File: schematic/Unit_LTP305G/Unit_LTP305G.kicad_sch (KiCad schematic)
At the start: 15 parts, among them J1 Conn_01x04, U1 M5StampS3, U2 LTP305G, U3 LTR305G

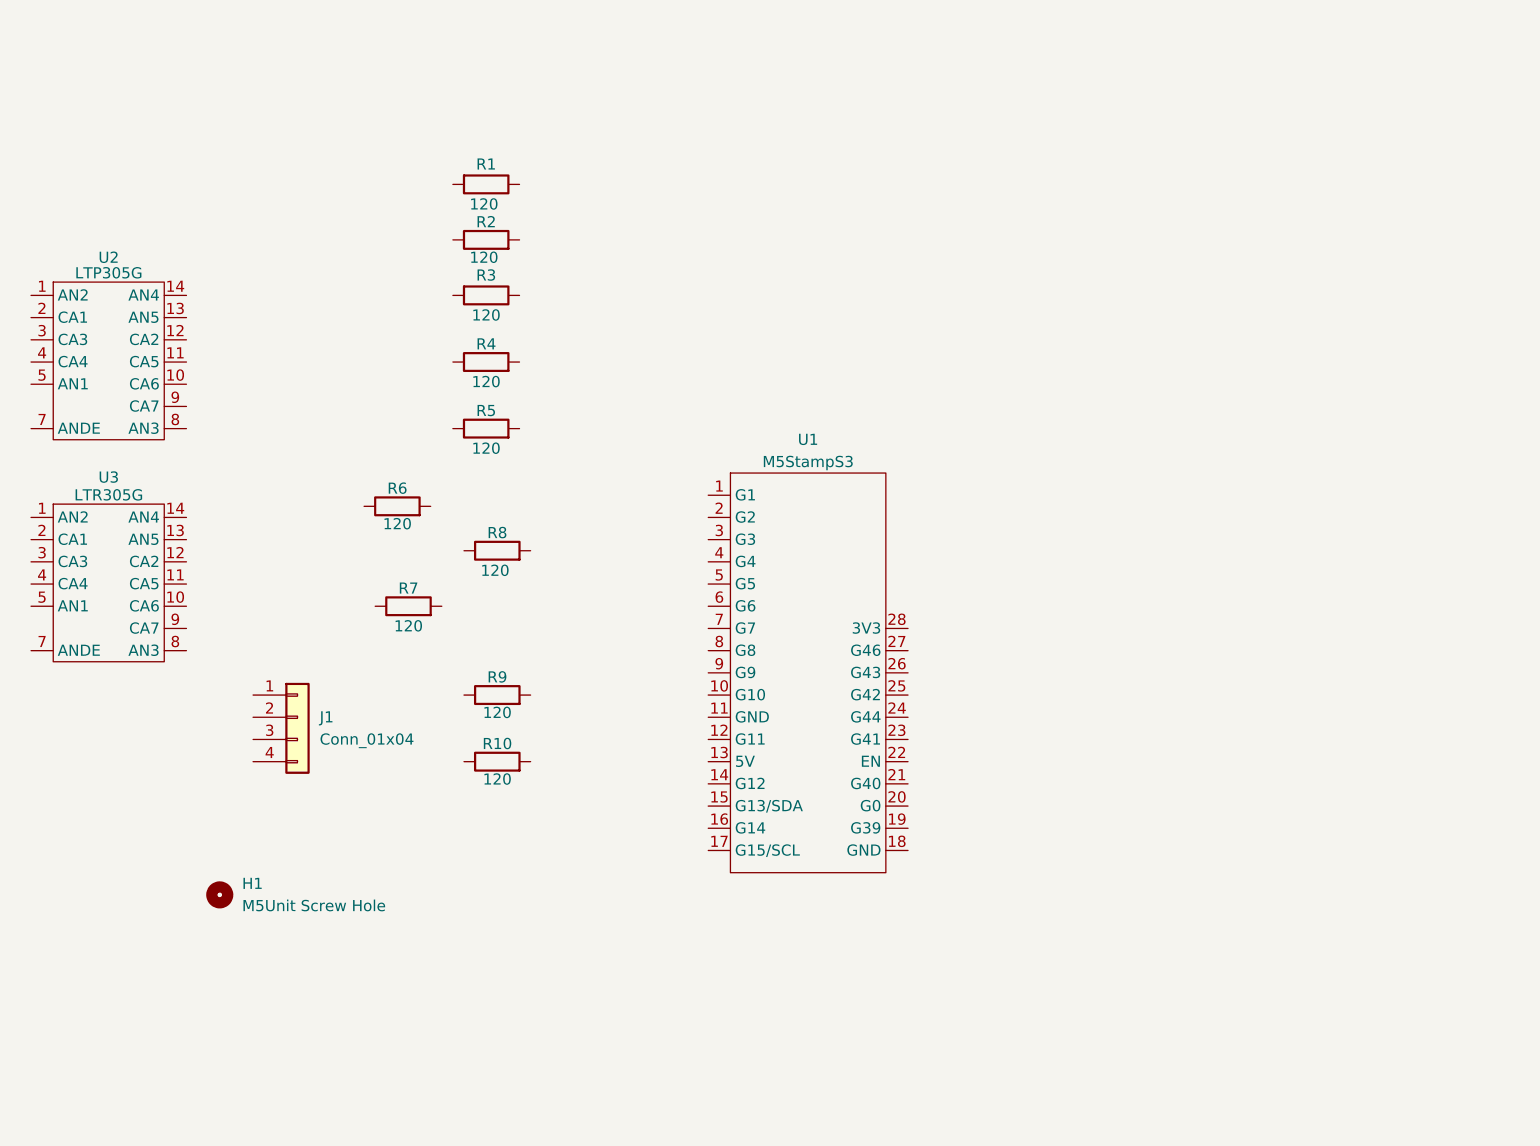
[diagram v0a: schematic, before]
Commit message: 基板設計
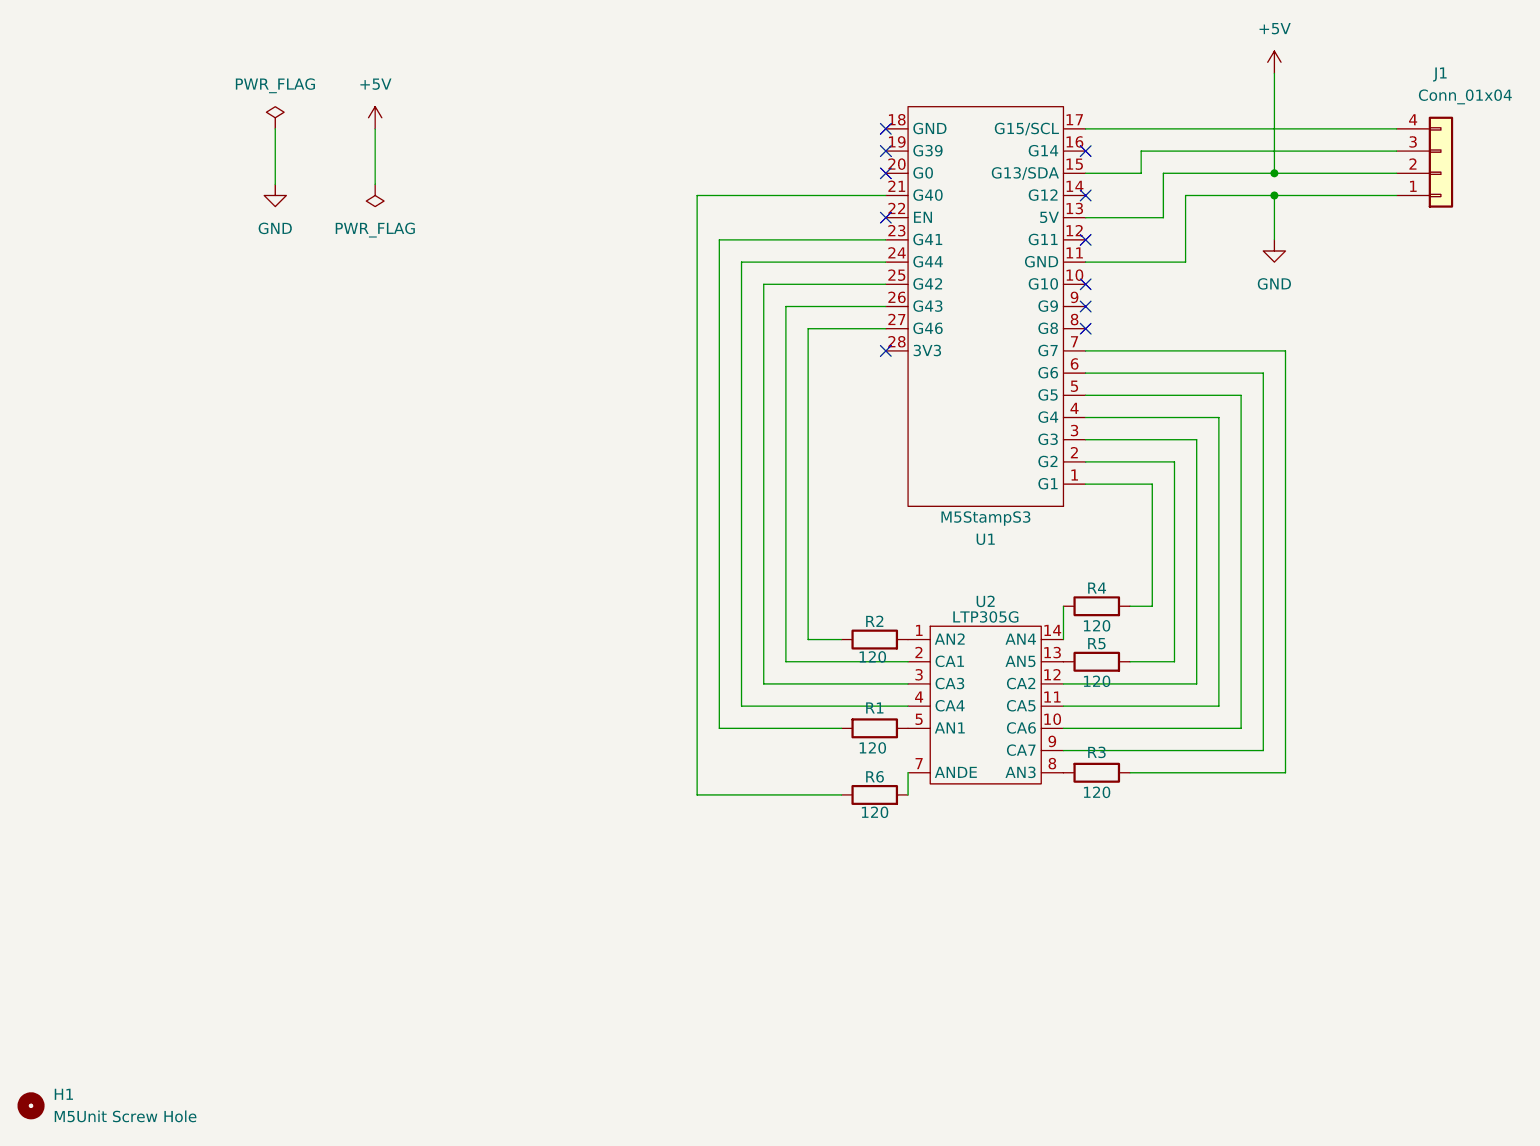
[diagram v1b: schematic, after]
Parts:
- removed R10, R7, R8, R9: 120, symbol Device:R
- removed U3: LTR305G, footprints:LTP305G, symbol Unit-HDPL:LTP3055G
- R1, R2, R3, R4, R5, R6: footprint (none) -> Resistor_SMD:R_0805_2012Metric_Pad1.20x1.40mm_HandSolder
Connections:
- net GND: now reaches J1.1 (Pin_1)
- net GND: now also U1.11 (GND)
- net +5V: now reaches J1.2 (Pin_2)
- net +5V: now also U1.13 (5V)
- net at J1.3 (Pin_3): now also U1.15 (G13/SDA)
- net at J1.4 (Pin_4): now also U1.17 (G15/SCL)
- net at R5.1: now also U2.13 (AN5)
- net at R5.2: now also U1.2 (G2)
- net at U1.1 (G1): now also R4.2
- net at U1.21 (G40): now also R6.1
- net at U1.23 (G41): now also R1.2
- net at U1.24 (G44): now also U2.4 (CA4)
- net at U1.25 (G42): now also U2.3 (CA3)
- net at U1.26 (G43): now also U2.2 (CA1)
- net at U1.27 (G46): now also R2.1
- net at U1.3 (G3): now also U2.12 (CA2)
- net at U1.4 (G4): now also U2.11 (CA5)
- net at U1.5 (G5): now also U2.10 (CA6)
- net at U1.6 (G6): now also U2.9 (CA7)
- net at U1.7 (G7): now also R3.1
- net at R4.1: now also U2.14 (AN4)
- net at R3.2: now also U2.8 (AN3)
- net at R2.2: now also U2.1 (AN2)
- net at R6.2: now also U2.7 (ANDE)
- net at R1.1: now also U2.5 (AN1)
- no-connect marks 0 -> 11
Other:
- moved on the sheet: H1, J1, R1, R2, R3, R4, R5, R6, U1, U2
